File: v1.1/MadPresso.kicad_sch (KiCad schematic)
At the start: 36 parts, among them J1 Conn_01x07, J2 Conn_01x03, J3 Conn_01x04, Q1 BSS84, Q3 BC847, U1 LTV-356T, U2 WeMos_D1_mini, U8 ADC101C021CIMK

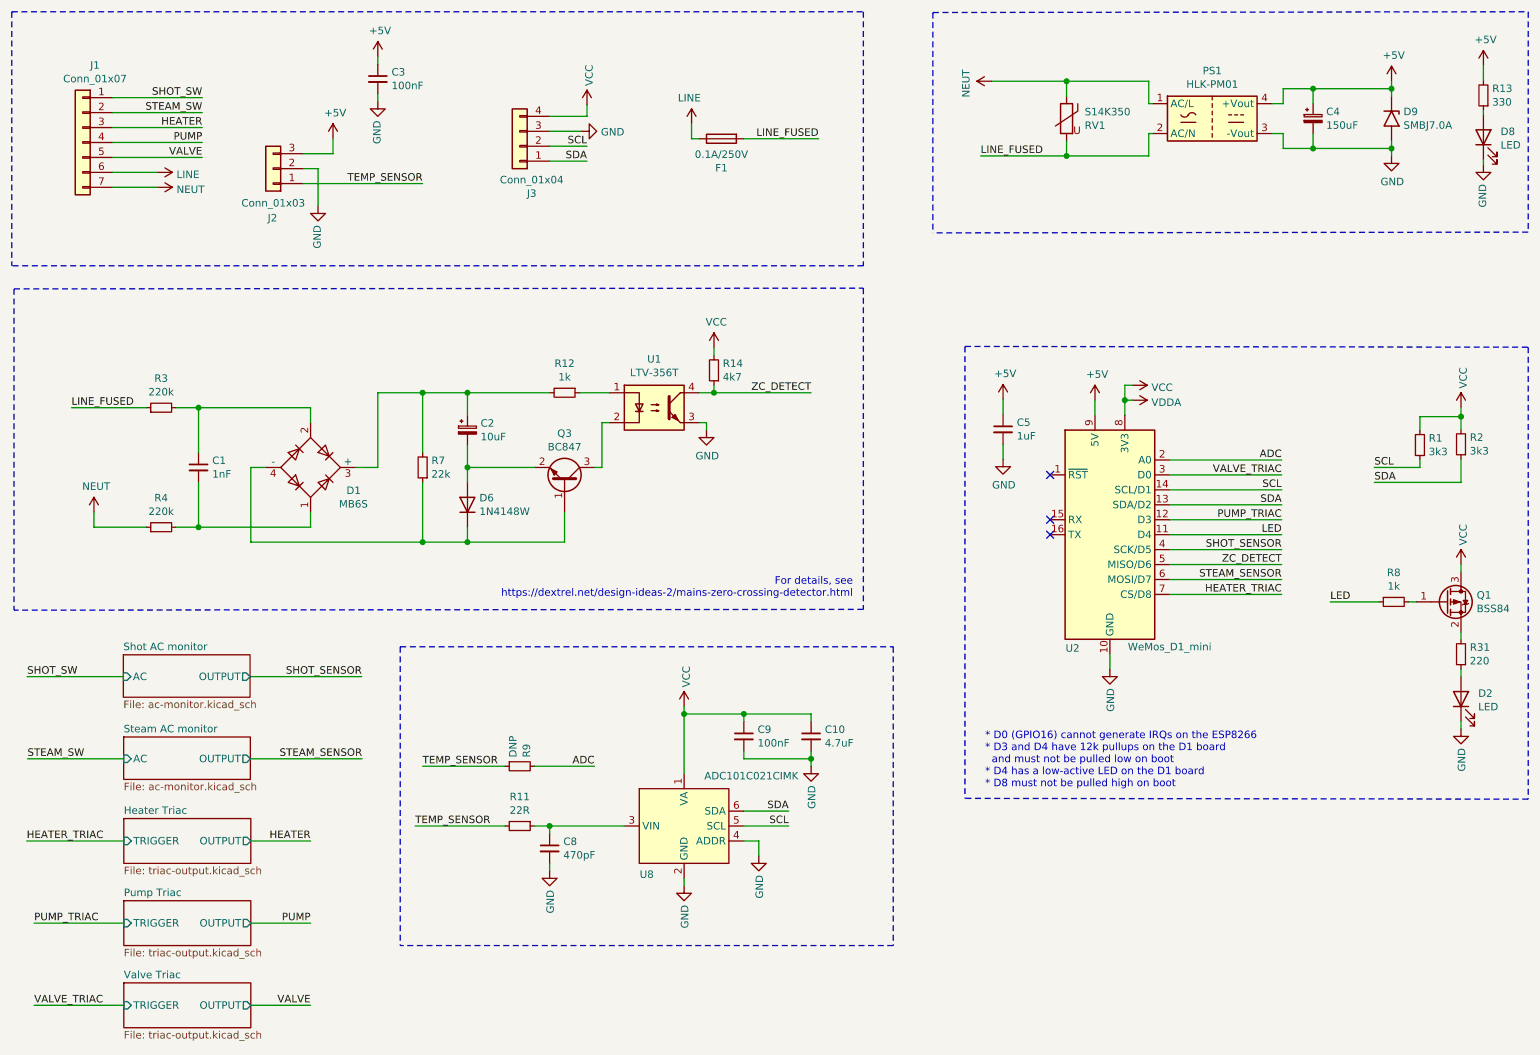
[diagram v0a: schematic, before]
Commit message: cleanups all over
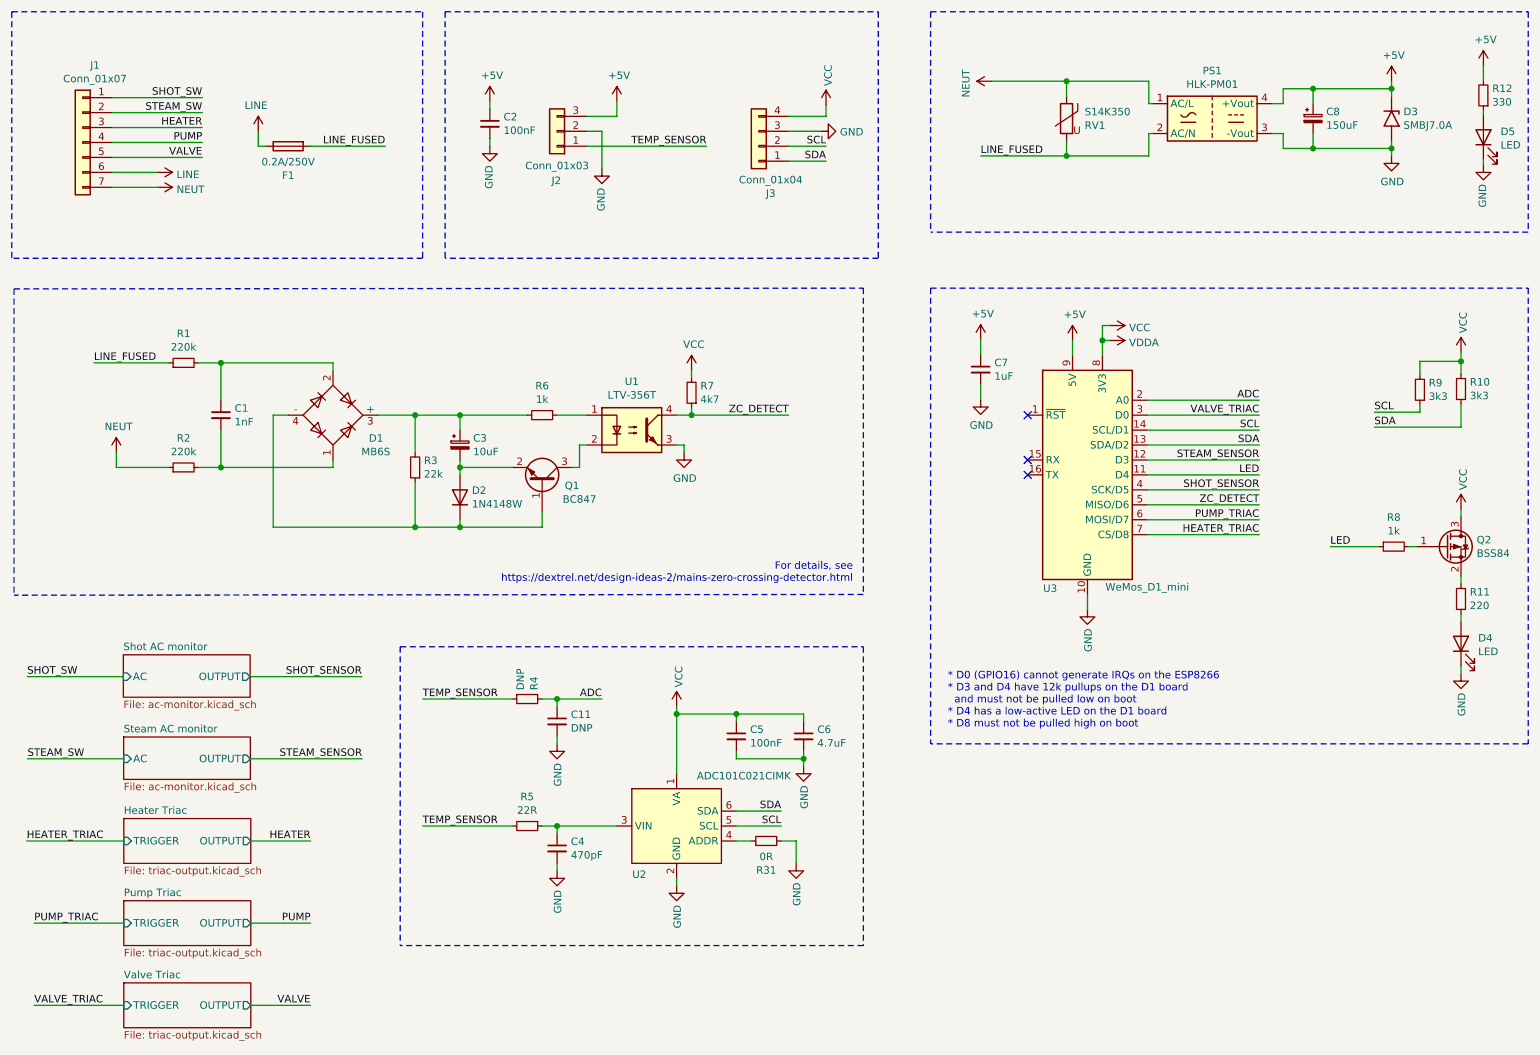
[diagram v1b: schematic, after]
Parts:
- added C11: DNP, Capacitor_SMD:C_0603_1608Metric_Pad1.08x0.95mm_HandSolder, symbol Device:C_Small
- added R31: 0R, Resistor_SMD:R_0603_1608Metric_Pad0.98x0.95mm_HandSolder, symbol Device:R_Small
- C1: footprint Capacitor_SMD:C_0603_1608Metric_Pad1.05x0.95mm_HandSolder -> Capacitor_SMD:C_0603_1608Metric_Pad1.08x0.95mm_HandSolder
- C2: renamed from C3; footprint Capacitor_SMD:C_0603_1608Metric_Pad1.05x0.95mm_HandSolder -> Capacitor_SMD:C_0603_1608Metric_Pad1.08x0.95mm_HandSolder
- C4: renamed from C8; footprint Capacitor_SMD:C_0603_1608Metric_Pad1.05x0.95mm_HandSolder -> Capacitor_SMD:C_0603_1608Metric_Pad1.08x0.95mm_HandSolder
- C5: renamed from C9; footprint Capacitor_SMD:C_0603_1608Metric_Pad1.05x0.95mm_HandSolder -> Capacitor_SMD:C_0603_1608Metric_Pad1.08x0.95mm_HandSolder
- C6: renamed from C10; footprint Capacitor_SMD:C_0603_1608Metric_Pad1.05x0.95mm_HandSolder -> Capacitor_SMD:C_0603_1608Metric_Pad1.08x0.95mm_HandSolder
- C7: renamed from C5; footprint Capacitor_SMD:C_0603_1608Metric_Pad1.05x0.95mm_HandSolder -> Capacitor_SMD:C_0603_1608Metric_Pad1.08x0.95mm_HandSolder
- F1: value 0.1A/250V -> 0.2A/250V
- R1: renamed from R3; footprint Resistor_SMD:R_1206_3216Metric_Pad1.42x1.75mm_HandSolder -> Resistor_SMD:R_1206_3216Metric_Pad1.30x1.75mm_HandSolder
- R10: renamed from R2; footprint Resistor_SMD:R_0603_1608Metric_Pad1.05x0.95mm_HandSolder -> Resistor_SMD:R_0603_1608Metric_Pad0.98x0.95mm_HandSolder
- R11: renamed from R31; footprint Resistor_SMD:R_0603_1608Metric_Pad1.05x0.95mm_HandSolder -> Resistor_SMD:R_0603_1608Metric_Pad0.98x0.95mm_HandSolder
- R12: renamed from R13; footprint Resistor_SMD:R_0603_1608Metric_Pad1.05x0.95mm_HandSolder -> Resistor_SMD:R_0603_1608Metric_Pad0.98x0.95mm_HandSolder
- R2: renamed from R4; footprint Resistor_SMD:R_1206_3216Metric_Pad1.42x1.75mm_HandSolder -> Resistor_SMD:R_1206_3216Metric_Pad1.30x1.75mm_HandSolder
- R3: renamed from R7; footprint Resistor_SMD:R_0603_1608Metric_Pad1.05x0.95mm_HandSolder -> Resistor_SMD:R_0603_1608Metric_Pad0.98x0.95mm_HandSolder
- R4: renamed from R9; footprint Resistor_SMD:R_0603_1608Metric_Pad1.05x0.95mm_HandSolder -> Resistor_SMD:R_0603_1608Metric_Pad0.98x0.95mm_HandSolder
- R5: renamed from R11; footprint Resistor_SMD:R_0603_1608Metric_Pad1.05x0.95mm_HandSolder -> Resistor_SMD:R_0603_1608Metric_Pad0.98x0.95mm_HandSolder
- R6: renamed from R12; footprint Resistor_SMD:R_0603_1608Metric_Pad1.05x0.95mm_HandSolder -> Resistor_SMD:R_0603_1608Metric_Pad0.98x0.95mm_HandSolder
- R7: renamed from R14; footprint Resistor_SMD:R_0603_1608Metric_Pad1.05x0.95mm_HandSolder -> Resistor_SMD:R_0603_1608Metric_Pad0.98x0.95mm_HandSolder
- R8: footprint Resistor_SMD:R_0603_1608Metric_Pad1.05x0.95mm_HandSolder -> Resistor_SMD:R_0603_1608Metric_Pad0.98x0.95mm_HandSolder
- R9: renamed from R1; footprint Resistor_SMD:R_0603_1608Metric_Pad1.05x0.95mm_HandSolder -> Resistor_SMD:R_0603_1608Metric_Pad0.98x0.95mm_HandSolder
- U2: renamed from U8; footprint Package_TO_SOT_SMD:SOT-23-6 -> Package_TO_SOT_SMD:SOT-23-6_Handsoldering
- renumbered C2 to C3, C4 to C8, D6 to D2, D9 to D3, D2 to D4, D8 to D5, Q3 to Q1, Q1 to Q2, U2 to U3
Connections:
- net ADC: now also C11.1
- net GND: now also C11.2, R31.2; no longer U2.4 (ADDR)
- net PUMP_TRIAC: now also U3.6 (MOSI/D7); no longer U3.12 (D3)
- net STEAM_SENSOR: now also U3.12 (D3); no longer U3.6 (MOSI/D7)
- new net: R31.1, U2.4 (ADDR)
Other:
- moved on the sheet: C1, C2, C3, C4, C5, C6, C7, D1, D2, D4, F1, J2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
